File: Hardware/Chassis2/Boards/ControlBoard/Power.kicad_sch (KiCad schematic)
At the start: 51 parts

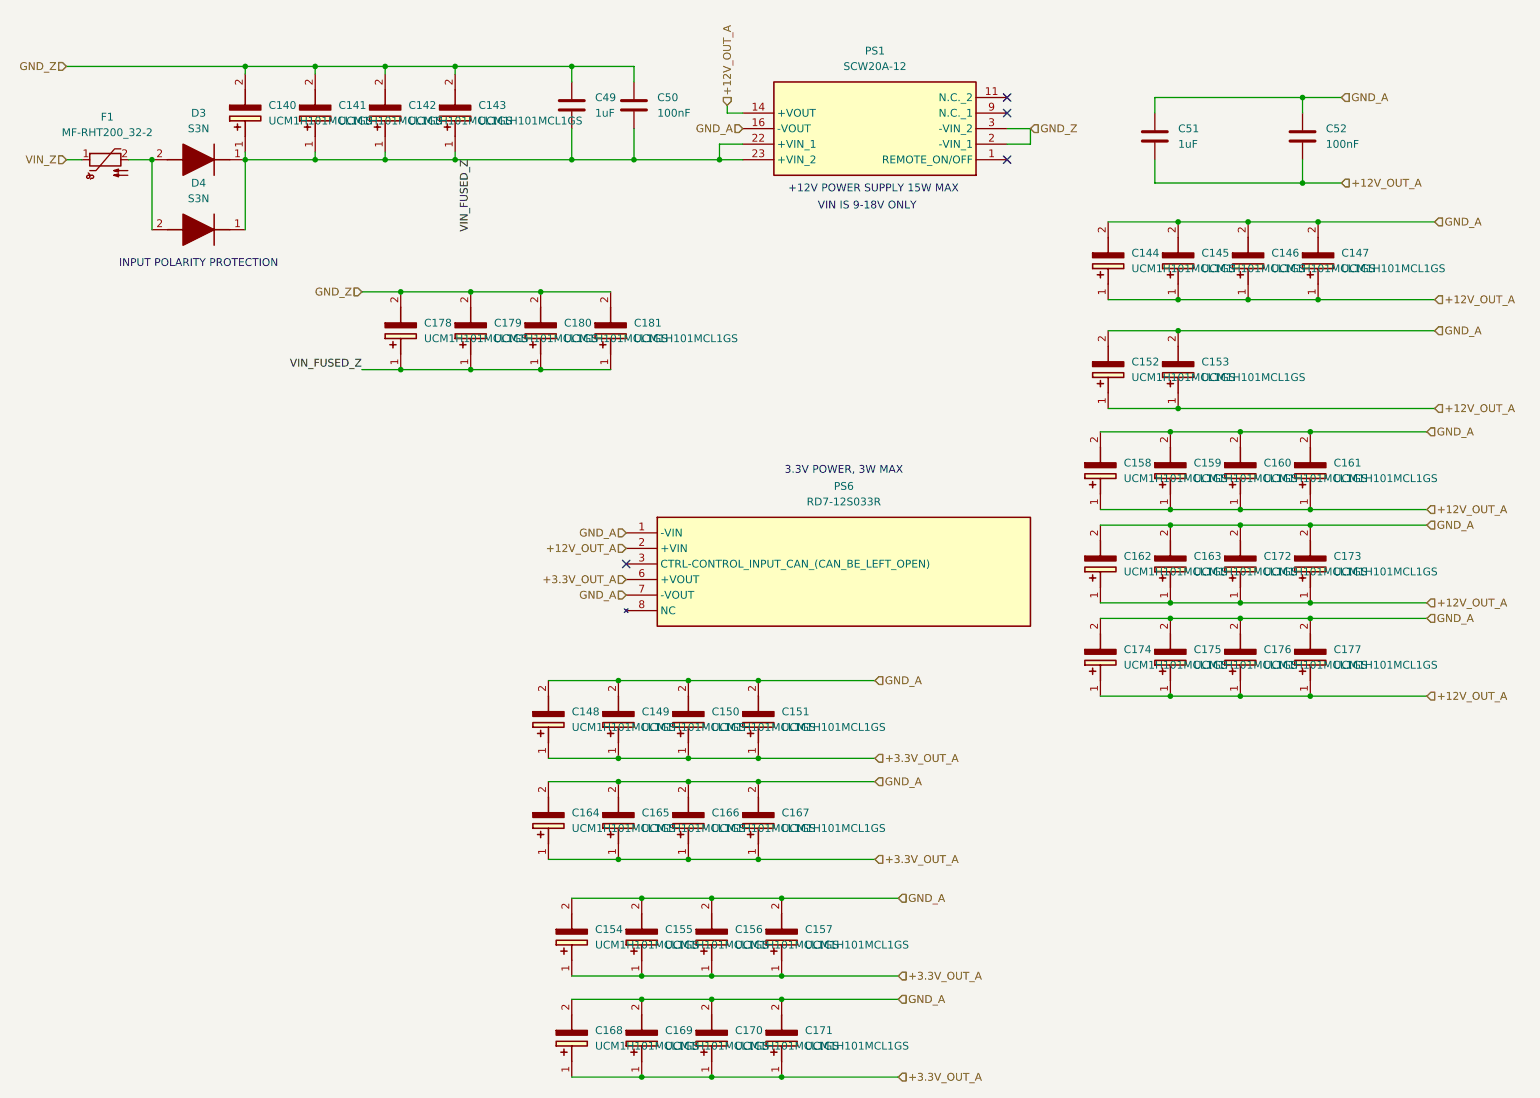
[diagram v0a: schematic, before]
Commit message: new stuff
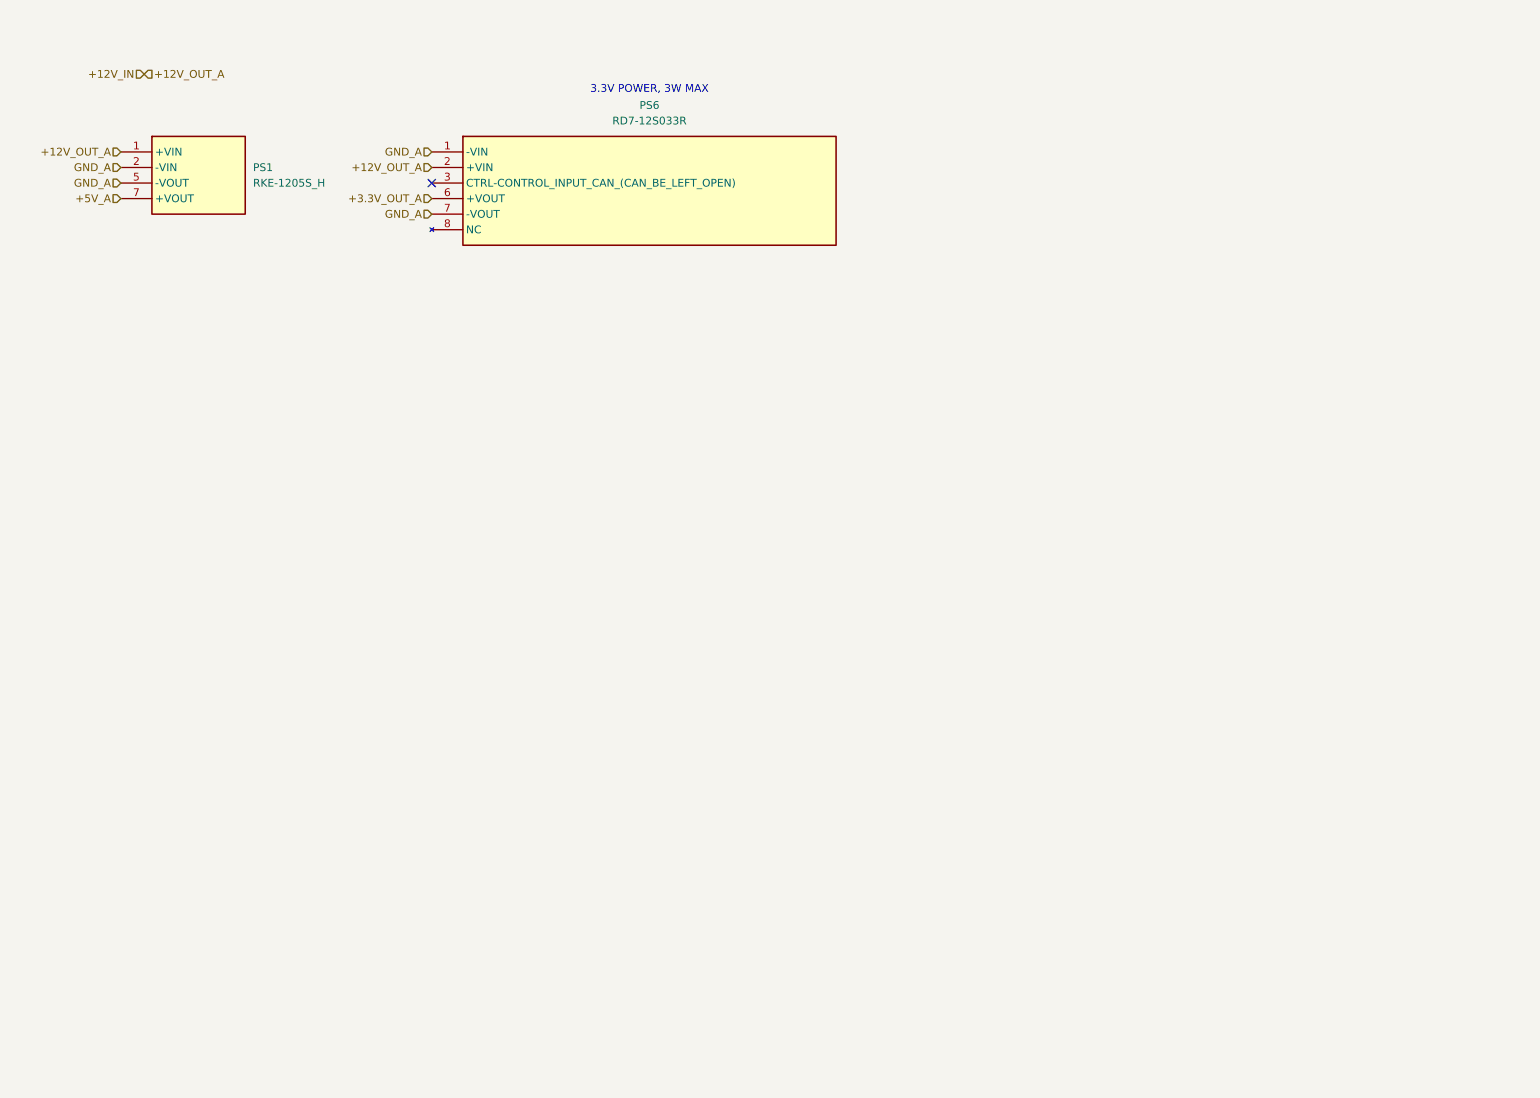
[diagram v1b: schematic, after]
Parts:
- removed C140, C141, C142, C143, C144, C145, C146, C147, C148, C149, C150, C151, C152, C153, C154, C155, C156, C157, C158, C159, C160, C161, C162, C163, C164, C165, C166, C167, C168, C169, C170, C171, C172, C173, C174, C175, C176, C177, C178, C179, C180, C181: UCM1H101MCL1GS, InverterCom:CAPAE660X800N, symbol InverterCom:UCM1H101MCL1GS
- removed C49, C51: 1uF, Capacitor_SMD:C_1210_3225Metric_Pad1.33x2.70mm_HandSolder, symbol Device:C
- removed C50, C52: 100nF, Capacitor_SMD:C_1210_3225Metric_Pad1.33x2.70mm_HandSolder, symbol Device:C
- removed D3, D4: S3N, InverterCom:DIOM8059X265N, symbol InverterCom:S3N
- removed F1: MF-RHT200_32-2, InverterCom:MFRHT200322, symbol InverterCom:MF-RHT200_32-2
- removed PS1: SCW20A-12, InverterCom:SCW20A12, symbol InverterCom:SCW20A-12
- added PS1: RKE-1205S_H, InverterCom:RKE1205SH, symbol InverterCom:RKE-1205S_H
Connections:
- net GND_A: now also PS1.2 (-VIN), PS1.5 (-VOUT)
- net +12V_OUT_A renamed +12V_IN
- net +12V_IN: now also PS1.1 (+VIN)
- new net +5V_A: PS1.7 (+VOUT)
- no-connect marks 4 -> 1
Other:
- note removed: "+12V POWER SUPPLY 15W MAX"
- note removed: "INPUT POLARITY PROTECTION"
- note removed: "VIN IS 9-18V ONLY"
- moved on the sheet: PS6
